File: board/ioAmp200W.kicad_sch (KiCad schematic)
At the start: 183 parts, among them J1 USB4105-GF-A-120, J2 USB4105-GF-A-120, J3 Speaker_Out, J4 SM03B-SRSS-TB, J5 5V_OUT, SW1 SW_Push, U1 RP2350_60QFN, U10 TPS7A1601DRBR, U11 LM70660RRXR, U12 TLV75733PDRVR, U14 MA5332MS, U15 TAD5112, U2 TPS26750SRSMR, U3 TPD4S480RUKR, U4 LP5912-3.3DRV, U5 MA5332MS, U6 SN74AHCT245RGYR, U7 SN74AHCT245RGYR, U8 Winbond W25Q32JVUUIQ, U9 TLV9162IDSGR, Y1 ABM8-272-T3

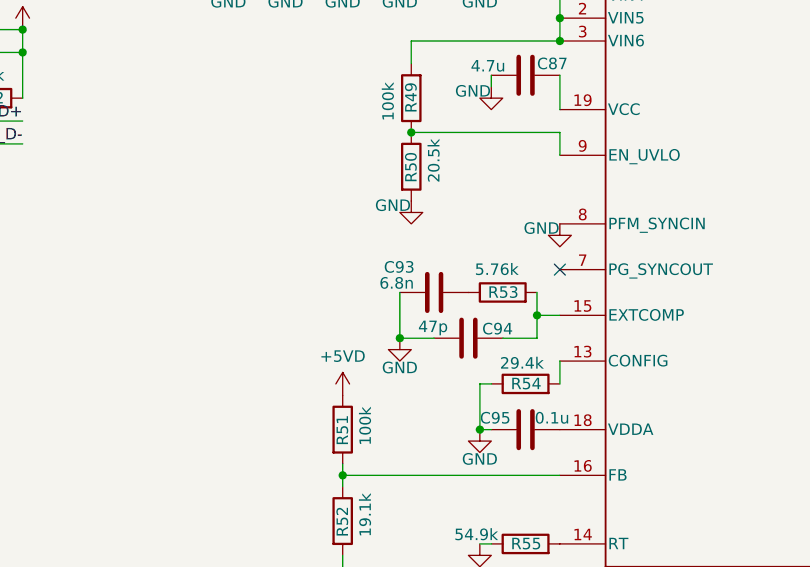
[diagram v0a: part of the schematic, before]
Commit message: verifybuck
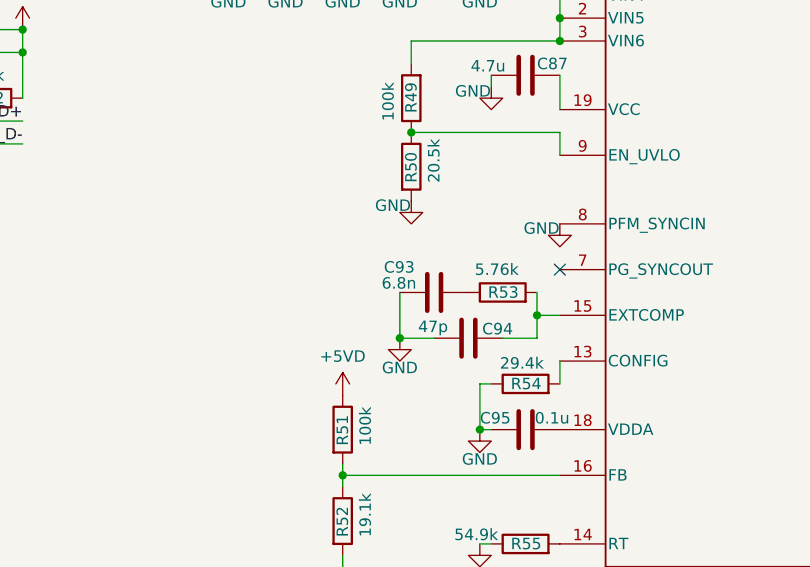
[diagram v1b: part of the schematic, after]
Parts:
- C83, C84, C85, C86: footprint Capacitor_SMD:C_0402_1005Metric -> Capacitor_SMD:C_1210_3225Metric; LCSC (none) -> C440151
- C87, C88, C89, C90: footprint Capacitor_SMD:C_0402_1005Metric -> Capacitor_SMD:C_1210_3225Metric; LCSC (none) -> C913445
- C91: footprint Capacitor_SMD:C_0402_1005Metric -> Capacitor_SMD:C_1210_3225Metric
- L4: footprint Capacitor_SMD:C_0402_1005Metric -> Inductor_SMD:L_Bourns_SRP7028A_7.3x6.6mm; LCSC (none) -> C3040366
- R48: footprint Resistor_SMD:R_0402_1005Metric -> Resistor_SMD:R_1206_3216Metric; LCSC (none) -> C6973817
- SW1: LCSC (none) -> C720477
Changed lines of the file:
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@@
 			)
 		)
-		(property "Footprint" "Capacitor_SMD:C_0402_1005Metric"
+		(property "Footprint" "Capacitor_SMD:C_1210_3225Metric"
 			(at 247.3452 74.93 0)
 			(hide yes)
@@
 			)
 		)
+		(property "LCSC" "C440151"
+			(at 246.38 71.12 90)
+			(hide yes)
+			(show_name no)
+			(do_not_autoplace no)
+			(effects
+				(font
+					(size 1.27 1.27)
+				)
+			)
+		)
 		(pin "2"
 		)
@@
 			)
 		)
-		(property "Footprint" "Resistor_SMD:R_0402_1005Metric"
+		(property "Footprint" "Resistor_SMD:R_1206_3216Metric"
 			(at 219.71 64.262 90)
 			(hide yes)
@@
 			)
 		)
+		(property "LCSC" "C6973817"
+			(at 219.71 66.04 90)
+			(hide yes)
+			(show_name no)
+			(do_not_autoplace no)
+			(effects
+				(font
+					(size 1.27 1.27)
+				)
+			)
+		)
 		(pin "2"
 		)
@@
 			)
 		)
-		(property "Footprint" "Capacitor_SMD:C_0402_1005Metric"
+		(property "Footprint" "Capacitor_SMD:C_1210_3225Metric"
 			(at 234.6452 74.93 0)
 			(hide yes)
@@
 			)
 		)
+		(property "LCSC" "C440151"
+			(at 233.68 71.12 90)
+			(hide yes)
+			(show_name no)
+			(do_not_autoplace no)
+			(effects
+				(font
+					(size 1.27 1.27)
+				)
+			)
+		)
 		(pin "2"
 		)
@@
 			)
 		)
-		(property "Footprint" "Capacitor_SMD:C_0402_1005Metric"
+		(property "Footprint" "Capacitor_SMD:C_1210_3225Metric"
 			(at 121.6152 50.8 0)
 			(hide yes)
@@
 			)
 		)
+		(property "LCSC" "C913445"
+			(at 120.65 46.99 90)
+			(hide yes)
+			(show_name no)
+			(do_not_autoplace no)
+			(effects
+				(font
+					(size 1.27 1.27)
+				)
+			)
+		)
 		(pin "2"
 		)
@@
 		)
 		(property "Value" "6.8n"
-			(at 124.714 85.344 90)
+			(at 124.968 85.344 90)
 			(show_name no)
 			(do_not_autoplace no)
@@
 			)
 		)
-		(property "Footprint" "Capacitor_SMD:C_0402_1005Metric"
+		(property "Footprint" "Capacitor_SMD:C_1210_3225Metric"
 			(at 115.2652 50.8 0)
 			(hide yes)
@@
 			)
 		)
+		(property "LCSC" "C913445"
+			(at 114.3 46.99 90)
+			(hide yes)
+			(show_name no)
+			(do_not_autoplace no)
+			(effects
+				(font
+					(size 1.27 1.27)
+				)
+			)
+		)
 		(pin "2"
 		)
@@
 			)
 		)
-		(property "Footprint" "Capacitor_SMD:C_0402_1005Metric"
+		(property "Footprint" "Inductor_SMD:L_Bourns_SRP7028A_7.3x6.6mm"
 			(at 207.01 66.04 0)
 			(hide yes)
@@
 			)
 		)
+		(property "LCSC" "C3040366"
+			(at 207.01 66.04 90)
+			(hide yes)
+			(show_name no)
+			(do_not_autoplace no)
+			(effects
+				(font
+					(size 1.27 1.27)
+				)
+			)
+		)
 		(pin "1"
 		)
@@
 			)
 		)
-		(property "Footprint" "Capacitor_SMD:C_0402_1005Metric"
+		(property "Footprint" "Capacitor_SMD:C_1210_3225Metric"
 			(at 108.9152 50.8 0)
 			(hide yes)
@@
 			)
 		)
+		(property "LCSC" "C913445"
+			(at 107.95 46.99 90)
+			(hide yes)
+			(show_name no)
+			(do_not_autoplace no)
+			(effects
+				(font
+					(size 1.27 1.27)
+				)
+			)
+		)
 		(pin "2"
 		)
@@
 			)
 		)
-		(property "Footprint" "Capacitor_SMD:C_0402_1005Metric"
+		(property "Footprint" "Capacitor_SMD:C_1210_3225Metric"
 			(at 228.2952 74.93 0)
 			(hide yes)
@@
 			)
 		)
+		(property "LCSC" "C440151"
+			(at 227.33 71.12 90)
+			(hide yes)
+			(show_name no)
+			(do_not_autoplace no)
+			(effects
+				(font
+					(size 1.27 1.27)
+				)
+			)
+		)
 		(pin "2"
 		)
@@
 			)
 		)
+		(property "LCSC" "C720477"
+			(at 158.115 416.56 90)
+			(hide yes)
+			(show_name no)
+			(do_not_autoplace no)
+			(effects
+				(font
+					(size 1.27 1.27)
+				)
+			)
+		)
 		(pin "1"
 		)
@@
 			)
 		)
-		(property "Footprint" "Capacitor_SMD:C_0402_1005Metric"
+		(property "Footprint" "Capacitor_SMD:C_1210_3225Metric"
 			(at 127.9652 50.8 0)
 			(hide yes)
@@
 			)
 		)
-		(property "Footprint" "Capacitor_SMD:C_0402_1005Metric"
+		(property "Footprint" "Capacitor_SMD:C_1210_3225Metric"
 			(at 137.16 63.1952 0)
 			(hide yes)
@@
 			)
 		)
+		(property "LCSC" "C913445"
+			(at 140.97 62.23 90)
+			(hide yes)
+			(show_name no)
+			(do_not_autoplace no)
+			(effects
+				(font
+					(size 1.27 1.27)
+				)
+			)
+		)
 		(pin "2"
 		)
@@
 			)
 		)
-		(property "Footprint" "Capacitor_SMD:C_0402_1005Metric"
+		(property "Footprint" "Capacitor_SMD:C_1210_3225Metric"
 			(at 240.9952 74.93 0)
 			(hide yes)
@@
 			(hide yes)
 			(show_name no)
+			(do_not_autoplace no)
+			(effects
+				(font
+					(size 1.27 1.27)
+				)
+			)
+		)
+		(property "LCSC" "C440151"
+			(at 240.03 71.12 90)
+			(hide yes)
+			(show_name no)
